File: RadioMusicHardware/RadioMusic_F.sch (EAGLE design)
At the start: 30 parts, among them X1 VERT_SD_CARD

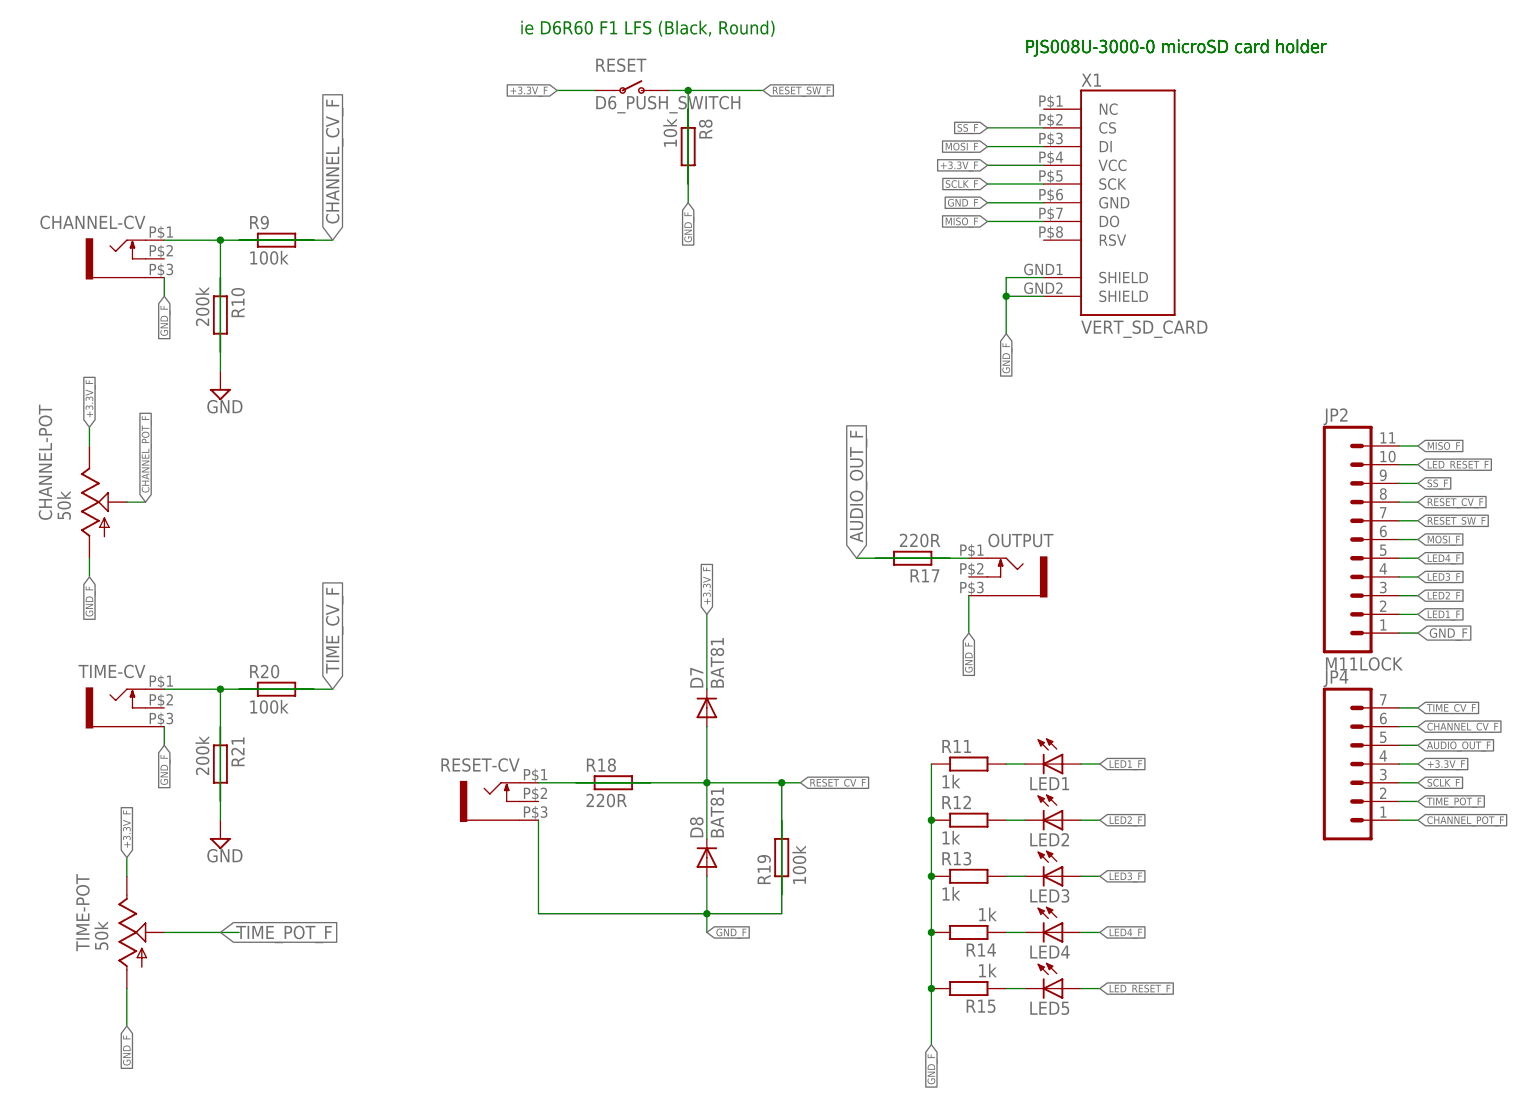
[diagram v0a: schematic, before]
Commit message: PCB cosmetic changes
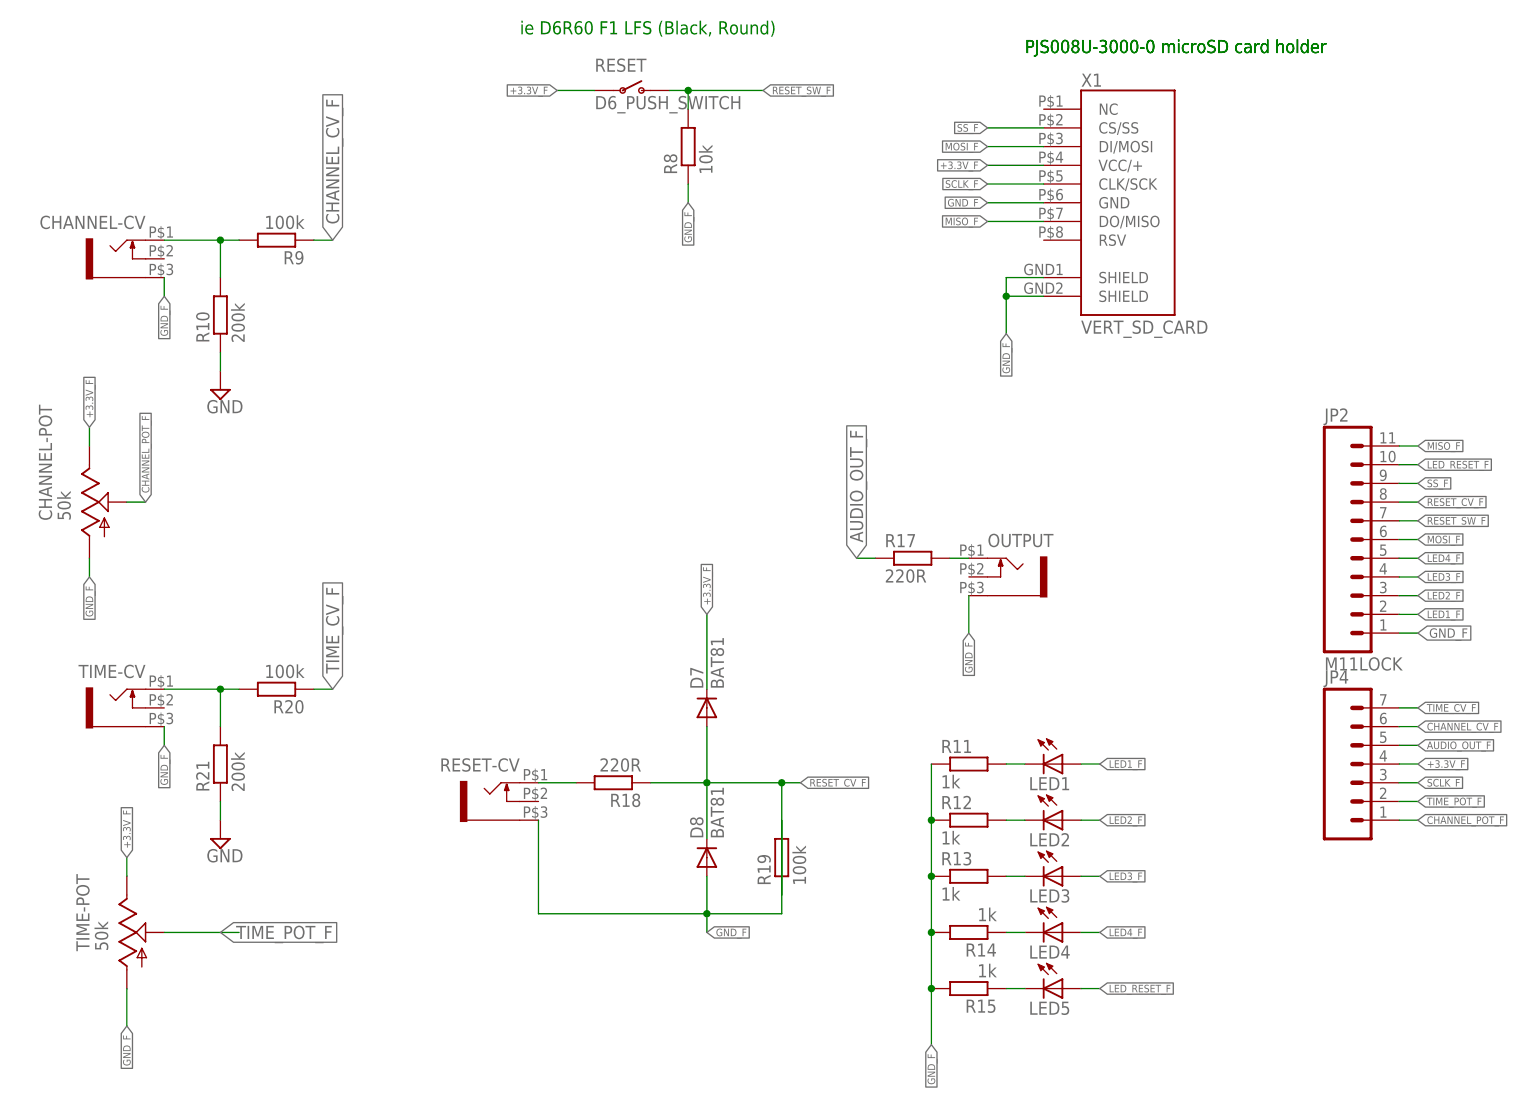
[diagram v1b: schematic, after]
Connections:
- net +3.3V_F: now also X1.VCC/+; no longer X1.VCC
- net MISO_F: now also X1.DO/MISO; no longer X1.DO
- net MOSI_F: now also X1.DI/MOSI; no longer X1.DI
- net SCLK_F: now also X1.CLK/SCK; no longer X1.SCK
- net SS_F: now also X1.CS/SS; no longer X1.CS
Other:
- moved on the sheet: R10, R17, R18, R20, R21, R8, R9
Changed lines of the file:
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@@
 <instance part="RESET-CV" gate="G$1" x="81.28" y="40.64" rot="MR0"/>
 <instance part="OUTPUT" gate="G$1" x="149.86" y="71.12"/>
-<instance part="R9" gate="G$1" x="50.8" y="116.84"/>
-<instance part="R10" gate="G$1" x="43.18" y="106.68" rot="R270"/>
+<instance part="R9" gate="G$1" x="50.8" y="116.84" rot="R180"/>
+<instance part="R10" gate="G$1" x="43.18" y="106.68" rot="R90"/>
 <instance part="SUPPLY4" gate="GND" x="43.18" y="96.52"/>
-<instance part="R17" gate="G$1" x="137.16" y="73.66" rot="R180"/>
+<instance part="R17" gate="G$1" x="137.16" y="73.66"/>
 <instance part="TIME-POT" gate="G$1" x="30.48" y="22.86"/>
 <instance part="TIME-CV" gate="G$1" x="30.48" y="53.34" rot="MR0"/>
-<instance part="R20" gate="G$1" x="50.8" y="55.88"/>
-<instance part="R21" gate="G$1" x="43.18" y="45.72" rot="R270"/>
+<instance part="R20" gate="G$1" x="50.8" y="55.88" rot="R180"/>
+<instance part="R21" gate="G$1" x="43.18" y="45.72" rot="R90"/>
 <instance part="SUPPLY5" gate="GND" x="43.18" y="35.56"/>
 <instance part="D7" gate="1" x="109.22" y="53.34" rot="R90"/>
 <instance part="D8" gate="1" x="109.22" y="33.02" rot="R90"/>
 <instance part="R19" gate="G$1" x="119.38" y="33.02" rot="R90"/>
-<instance part="R18" gate="G$1" x="96.52" y="43.18"/>
+<instance part="R18" gate="G$1" x="96.52" y="43.18" rot="R180"/>
 <instance part="RESET" gate="G$1" x="99.06" y="137.16"/>
-<instance part="R8" gate="G$1" x="106.68" y="129.54" rot="R270"/>
+<instance part="R8" gate="G$1" x="106.68" y="129.54" rot="R90"/>
 <instance part="LED1" gate="G$1" x="157.48" y="45.72" rot="R270"/>
 <instance part="LED2" gate="G$1" x="157.48" y="38.1" rot="R270"/>
@@
 <segment>
 <pinref part="R10" gate="G$1" pin="1"/>
-<wire x1="43.18" y1="111.76" x2="43.18" y2="99.06" width="0.1524" layer="91"/>
+<wire x1="43.18" y1="101.6" x2="43.18" y2="99.06" width="0.1524" layer="91"/>
 <pinref part="SUPPLY4" gate="GND" pin="GND"/>
 </segment>
 <segment>
 <pinref part="R21" gate="G$1" pin="1"/>
-<wire x1="43.18" y1="50.8" x2="43.18" y2="38.1" width="0.1524" layer="91"/>
+<wire x1="43.18" y1="40.64" x2="43.18" y2="38.1" width="0.1524" layer="91"/>
 <pinref part="SUPPLY5" gate="GND" pin="GND"/>
 </segment>
@@
 <pinref part="R18" gate="G$1" pin="2"/>
 <pinref part="RESET-CV" gate="G$1" pin="2"/>
-<wire x1="101.6" y1="43.18" x2="86.36" y2="43.18" width="0.1524" layer="91"/>
+<wire x1="91.44" y1="43.18" x2="86.36" y2="43.18" width="0.1524" layer="91"/>
 </segment>
 </net>
@@
 <net name="MISO_F" class="0">
 <segment>
-<pinref part="X1" gate="G$1" pin="DO"/>
+<pinref part="X1" gate="G$1" pin="DO/MISO"/>
 <wire x1="147.32" y1="119.38" x2="154.94" y2="119.38" width="0.1524" layer="91"/>
 <label x="147.32" y="119.38" size="1.016" layer="95" rot="R180" xref="yes"/>
@@
 <segment>
 <pinref part="R17" gate="G$1" pin="1"/>
-<wire x1="129.54" y1="73.66" x2="142.24" y2="73.66" width="0.1524" layer="91"/>
+<wire x1="129.54" y1="73.66" x2="132.08" y2="73.66" width="0.1524" layer="91"/>
 <label x="129.54" y="73.66" size="1.778" layer="95" rot="R90" xref="yes"/>
 </segment>
@@
 <pinref part="R8" gate="G$1" pin="2"/>
 <wire x1="106.68" y1="137.16" x2="116.84" y2="137.16" width="0.1524" layer="91"/>
-<wire x1="106.68" y1="124.46" x2="106.68" y2="137.16" width="0.1524" layer="91"/>
+<wire x1="106.68" y1="134.62" x2="106.68" y2="137.16" width="0.1524" layer="91"/>
 <junction x="106.68" y="137.16"/>
 <label x="116.84" y="137.16" size="1.016" layer="95" xref="yes"/>
@@
 <net name="+3.3V_F" class="0">
 <segment>
-<pinref part="X1" gate="G$1" pin="VCC"/>
+<pinref part="X1" gate="G$1" pin="VCC/+"/>
 <wire x1="147.32" y1="127" x2="154.94" y2="127" width="0.1524" layer="91"/>
 <label x="147.32" y="127" size="1.016" layer="95" rot="R180" xref="yes"/>
@@
 <segment>
 <pinref part="R8" gate="G$1" pin="1"/>
-<wire x1="106.68" y1="121.92" x2="106.68" y2="134.62" width="0.1524" layer="91"/>
+<wire x1="106.68" y1="121.92" x2="106.68" y2="124.46" width="0.1524" layer="91"/>
 <label x="106.68" y="121.92" size="1.016" layer="95" rot="R270" xref="yes"/>
 </segment>
@@
 <segment>
 <pinref part="R9" gate="G$1" pin="1"/>
-<wire x1="58.42" y1="116.84" x2="45.72" y2="116.84" width="0.1524" layer="91"/>
+<wire x1="58.42" y1="116.84" x2="55.88" y2="116.84" width="0.1524" layer="91"/>
 <label x="58.42" y="116.84" size="1.778" layer="95" rot="R90" xref="yes"/>
 </segment>
@@
 <segment>
 <pinref part="R20" gate="G$1" pin="1"/>
-<wire x1="58.42" y1="55.88" x2="45.72" y2="55.88" width="0.1524" layer="91"/>
+<wire x1="58.42" y1="55.88" x2="55.88" y2="55.88" width="0.1524" layer="91"/>
 <label x="58.42" y="55.88" size="1.778" layer="95" rot="R90" xref="yes"/>
 </segment>
@@
 <pinref part="R18" gate="G$1" pin="1"/>
 <wire x1="109.22" y1="43.18" x2="109.22" y2="50.8" width="0.1524" layer="91"/>
-<wire x1="91.44" y1="43.18" x2="109.22" y2="43.18" width="0.1524" layer="91"/>
+<wire x1="101.6" y1="43.18" x2="109.22" y2="43.18" width="0.1524" layer="91"/>
 <junction x="109.22" y="43.18"/>
 <wire x1="109.22" y1="43.18" x2="119.38" y2="43.18" width="0.1524" layer="91"/>
@@
 <net name="SCLK_F" class="0">
 <segment>
-<pinref part="X1" gate="G$1" pin="SCK"/>
+<pinref part="X1" gate="G$1" pin="CLK/SCK"/>
 <wire x1="147.32" y1="124.46" x2="154.94" y2="124.46" width="0.1524" layer="91"/>
 <label x="147.32" y="124.46" size="1.016" layer="95" rot="R180" xref="yes"/>
@@
 <net name="MOSI_F" class="0">
 <segment>
-<pinref part="X1" gate="G$1" pin="DI"/>
+<pinref part="X1" gate="G$1" pin="DI/MOSI"/>
 <wire x1="147.32" y1="129.54" x2="154.94" y2="129.54" width="0.1524" layer="91"/>
 <label x="147.32" y="129.54" size="1.016" layer="95" rot="R180" xref="yes"/>
@@
 <net name="SS_F" class="0">
 <segment>
-<pinref part="X1" gate="G$1" pin="CS"/>
+<pinref part="X1" gate="G$1" pin="CS/SS"/>
 <wire x1="147.32" y1="132.08" x2="154.94" y2="132.08" width="0.1524" layer="91"/>
 <label x="147.32" y="132.08" size="1.016" layer="95" rot="R180" xref="yes"/>
@@
 <segment>
 <pinref part="R20" gate="G$1" pin="2"/>
-<wire x1="55.88" y1="55.88" x2="43.18" y2="55.88" width="0.1524" layer="91"/>
+<wire x1="45.72" y1="55.88" x2="43.18" y2="55.88" width="0.1524" layer="91"/>
 <pinref part="R21" gate="G$1" pin="2"/>
 <wire x1="43.18" y1="55.88" x2="35.56" y2="55.88" width="0.1524" layer="91"/>
-<wire x1="43.18" y1="40.64" x2="43.18" y2="55.88" width="0.1524" layer="91"/>
+<wire x1="43.18" y1="50.8" x2="43.18" y2="55.88" width="0.1524" layer="91"/>
 <junction x="43.18" y="55.88"/>
 <pinref part="TIME-CV" gate="G$1" pin="2"/>
@@
 <pinref part="R9" gate="G$1" pin="2"/>
 <pinref part="CHANNEL-CV" gate="G$1" pin="2"/>
-<wire x1="55.88" y1="116.84" x2="43.18" y2="116.84" width="0.1524" layer="91"/>
+<wire x1="45.72" y1="116.84" x2="43.18" y2="116.84" width="0.1524" layer="91"/>
 <pinref part="R10" gate="G$1" pin="2"/>
 <wire x1="43.18" y1="116.84" x2="35.56" y2="116.84" width="0.1524" layer="91"/>
-<wire x1="43.18" y1="101.6" x2="43.18" y2="116.84" width="0.1524" layer="91"/>
+<wire x1="43.18" y1="111.76" x2="43.18" y2="116.84" width="0.1524" layer="91"/>
 <junction x="43.18" y="116.84"/>
 </segment>
@@
 <pinref part="OUTPUT" gate="G$1" pin="2"/>
 <pinref part="R17" gate="G$1" pin="2"/>
-<wire x1="132.08" y1="73.66" x2="144.78" y2="73.66" width="0.1524" layer="91"/>
-</segment>
-</net>
+<wire x1="142.24" y1="73.66" x2="144.78" y2="73.66" width="0.1524" layer="91"/>
+</segment>
+</net>

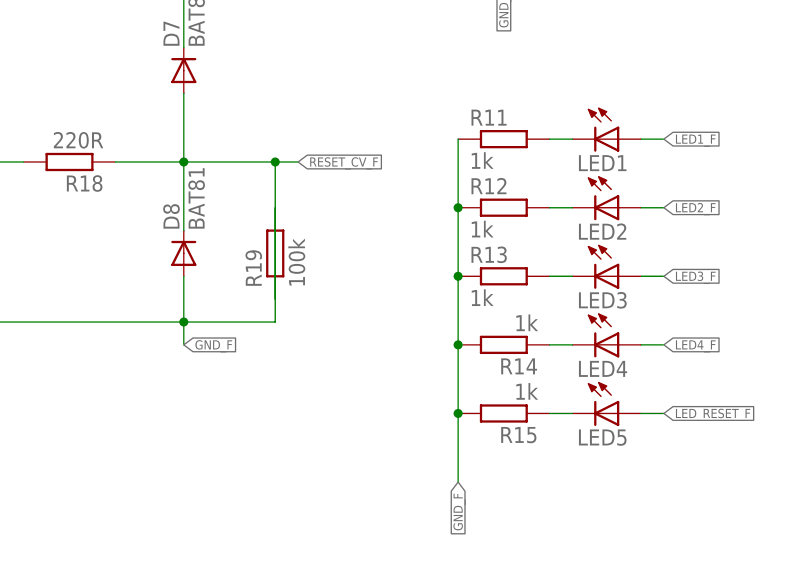
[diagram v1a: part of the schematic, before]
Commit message: Text subbing
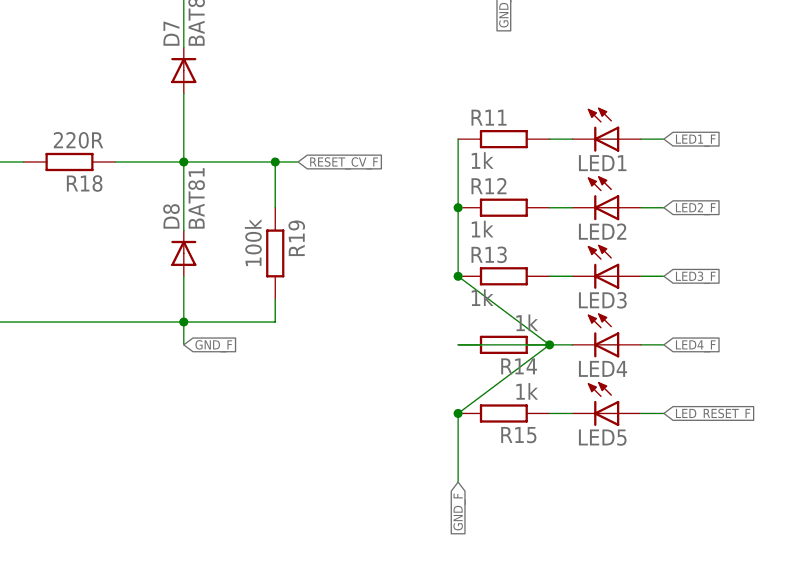
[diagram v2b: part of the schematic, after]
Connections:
- net GND_F: now also R14.1; no longer R14.2
- net N$21: now also R14.2; no longer R14.1
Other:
- moved on the sheet: R19
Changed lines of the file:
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@@
 <instance part="D7" gate="1" x="109.22" y="53.34" rot="R90"/>
 <instance part="D8" gate="1" x="109.22" y="33.02" rot="R90"/>
-<instance part="R19" gate="G$1" x="119.38" y="33.02" rot="R90"/>
+<instance part="R19" gate="G$1" x="119.38" y="33.02" rot="R270"/>
 <instance part="R18" gate="G$1" x="96.52" y="43.18" rot="R180"/>
 <instance part="RESET" gate="G$1" x="99.06" y="137.16"/>
@@
 <segment>
 <pinref part="LED4" gate="G$1" pin="C"/>
-<pinref part="R14" gate="G$1" pin="1"/>
-<wire x1="149.86" y1="22.86" x2="152.4" y2="22.86" width="0.1524" layer="91"/>
+<pinref part="R14" gate="G$1" pin="2"/>
+<wire x1="139.7" y1="22.86" x2="152.4" y2="22.86" width="0.1524" layer="91"/>
 </segment>
 </net>
@@
 <wire x1="86.36" y1="38.1" x2="86.36" y2="25.4" width="0.1524" layer="91"/>
 <pinref part="R19" gate="G$1" pin="2"/>
-<wire x1="119.38" y1="38.1" x2="119.38" y2="25.4" width="0.1524" layer="91"/>
+<wire x1="119.38" y1="27.94" x2="119.38" y2="25.4" width="0.1524" layer="91"/>
 <pinref part="D8" gate="1" pin="A"/>
 <wire x1="109.22" y1="25.4" x2="109.22" y2="30.48" width="0.1524" layer="91"/>
@@
 <junction x="139.7" y="38.1"/>
 <pinref part="R13" gate="G$1" pin="1"/>
-<wire x1="139.7" y1="30.48" x2="139.7" y2="22.86" width="0.1524" layer="91"/>
+<wire x1="139.7" y1="30.48" x2="149.86" y2="22.86" width="0.1524" layer="91"/>
 <junction x="139.7" y="30.48"/>
-<pinref part="R14" gate="G$1" pin="2"/>
-<wire x1="139.7" y1="22.86" x2="139.7" y2="15.24" width="0.1524" layer="91"/>
-<junction x="139.7" y="22.86"/>
+<pinref part="R14" gate="G$1" pin="1"/>
+<wire x1="149.86" y1="22.86" x2="139.7" y2="15.24" width="0.1524" layer="91"/>
+<junction x="149.86" y="22.86"/>
 <pinref part="R15" gate="G$1" pin="2"/>
 <wire x1="139.7" y1="15.24" x2="139.7" y2="7.62" width="0.1524" layer="91"/>
@@
 <pinref part="R19" gate="G$1" pin="1"/>
 <wire x1="119.38" y1="43.18" x2="121.92" y2="43.18" width="0.1524" layer="91"/>
-<wire x1="119.38" y1="27.94" x2="119.38" y2="43.18" width="0.1524" layer="91"/>
+<wire x1="119.38" y1="38.1" x2="119.38" y2="43.18" width="0.1524" layer="91"/>
 <junction x="119.38" y="43.18"/>
 <label x="121.92" y="43.18" size="1.016" layer="95" xref="yes"/>
